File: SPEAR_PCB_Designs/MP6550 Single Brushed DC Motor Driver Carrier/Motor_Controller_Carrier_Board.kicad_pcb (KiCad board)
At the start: 2 copper layers, 104 x 47 mm, 21 parts, among them J1 Conn_01x02_Pin, J2 Conn_01x02_Pin, J3 Conn_01x02_Pin, J4 Conn_01x04_Pin, U1 AP63203WU

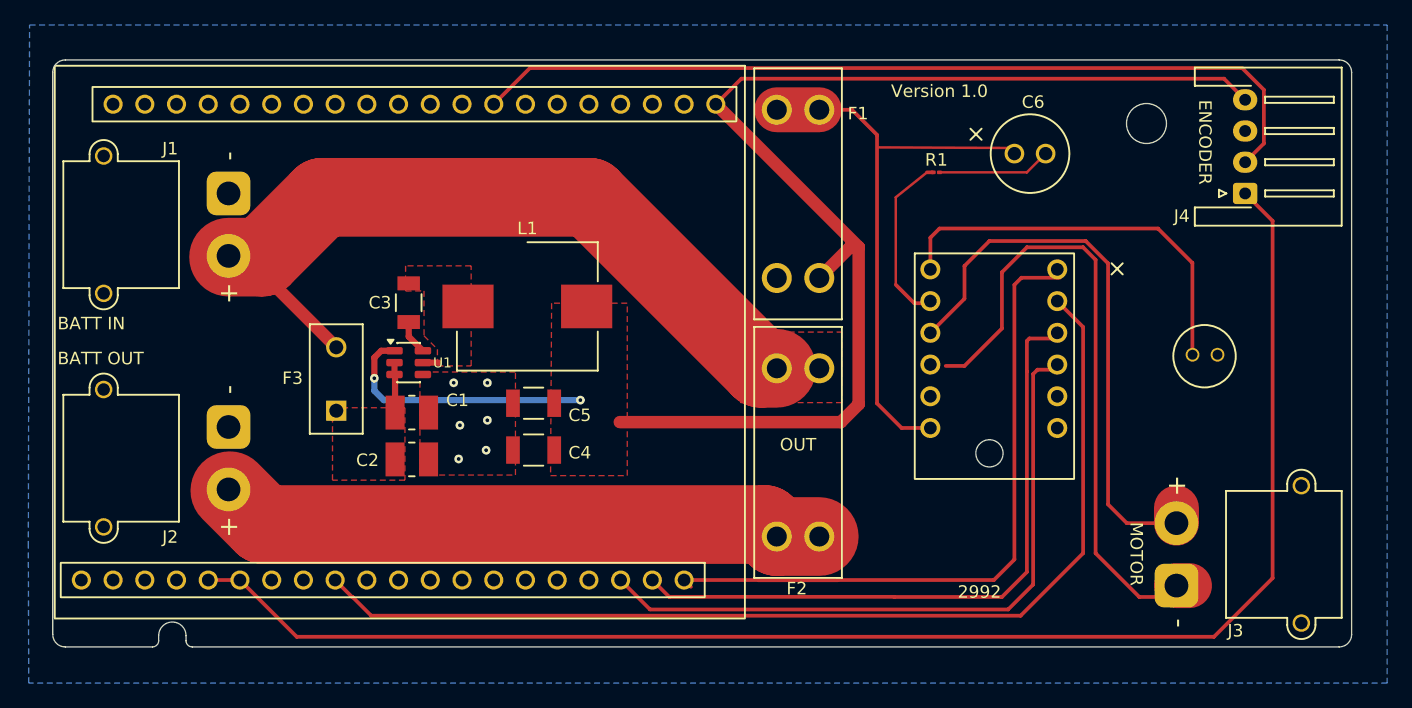
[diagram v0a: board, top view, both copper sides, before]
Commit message: update
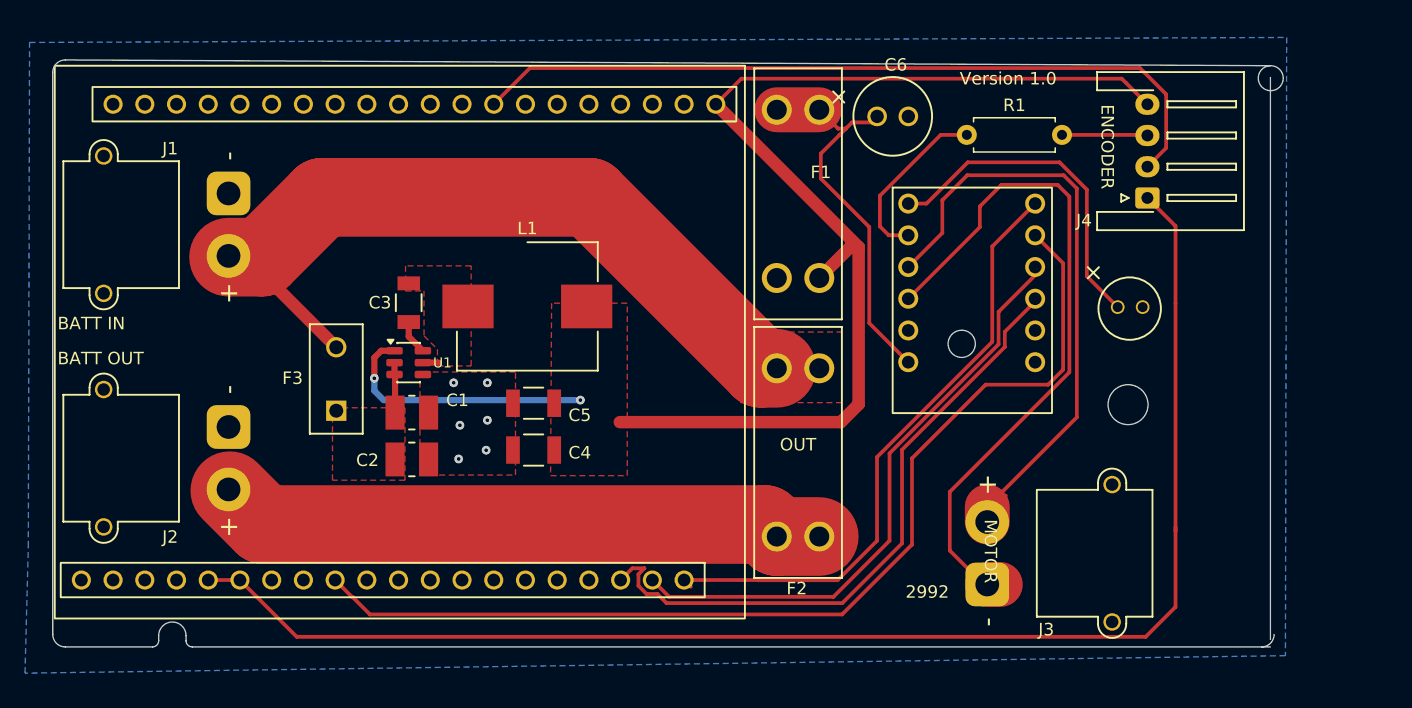
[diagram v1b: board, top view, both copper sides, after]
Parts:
- R1: footprint Resistor_SMD:R_01005_0402Metric -> Resistor_THT:R_Axial_DIN0207_L6.3mm_D2.5mm_P7.62mm_Horizontal
- moved REF** 22.6 mm to (171.1, 96.6)
- moved J3 15.2 mm to (159.8, 111.0)
- moved C6 11.4 mm to (148.5, 73.5)
- moved J4 7.83 mm to (172.7, 80.0)
- moved C7 7.10 mm to (173.4, 88.8)
- moved MDB1 5.56 mm to (152.2, 79.2)
- moved R1 3.87 mm to (158.2, 75.0)
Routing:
- net Net-(MDB1-ISET): track 4.20 -> 14.3 mm
- net +3.3V: track 117.7 -> 110.0 mm
- net /Schematic/ENC_A: track 70.0 -> 62.3 mm
- net GND: track 0.00 -> 6.86 mm
- net /Schematic/ENC_B: track 120.8 -> 114.4 mm
- net Net-(J3-Pin_1): track 51.8 -> 57.6 mm
- net Net-(MDB1-V3P3): track 32.7 -> 27.0 mm
- net Net-(J3-Pin_2): track 46.5 -> 51.4 mm
- net Net-(MDB1-VIN): track 35.4 -> 31.5 mm
- net /Schematic/PWM2: track 52.6 -> 48.8 mm
- net /Schematic/GPIO: track 53.8 -> 50.7 mm
- net /Schematic/PWM1: track 53.9 -> 51.4 mm
- net /Schematic/ADC: track 84.2 -> 83.3 mm
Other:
- board size 104 x 47 mm -> 98.5 x 47 mm

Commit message: updates
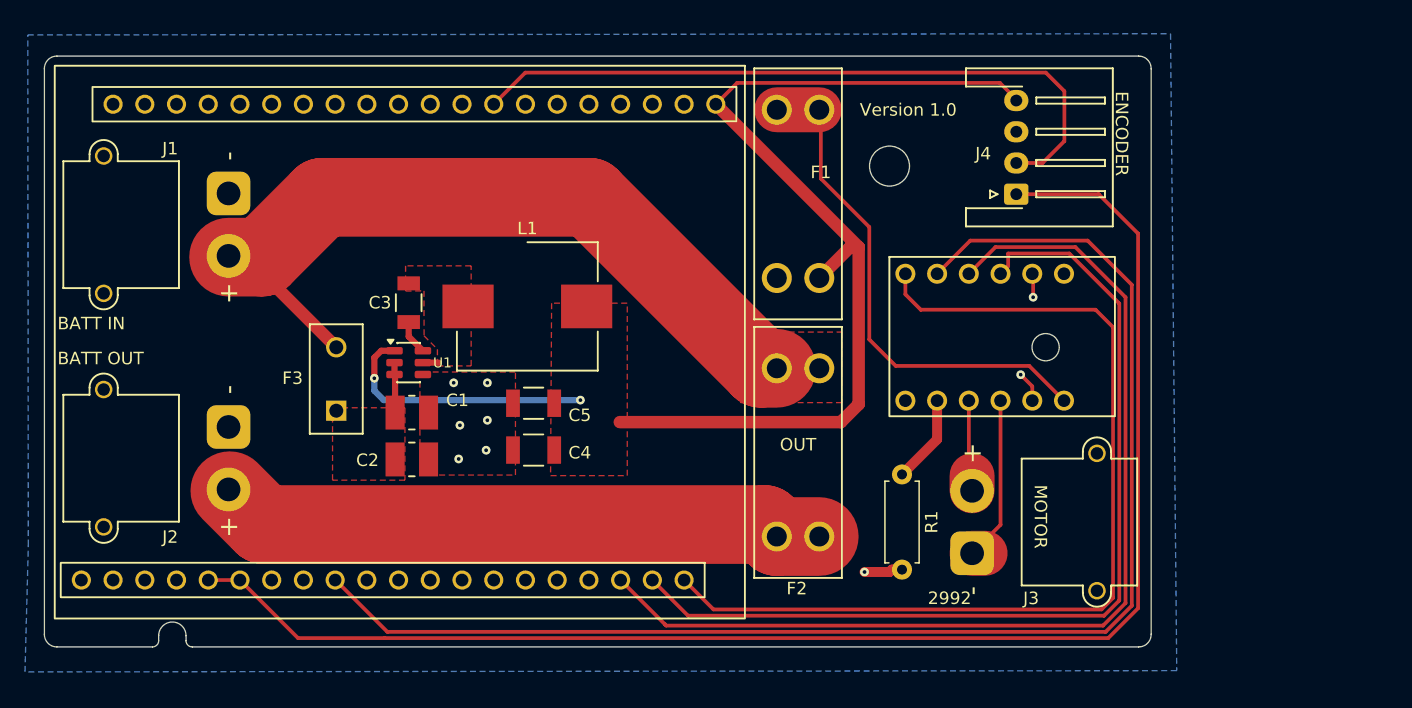
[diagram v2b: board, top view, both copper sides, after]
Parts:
- removed C6: 47uF, Motor_Controller_Carrier_Board:CAP_UBY_6.3X11_NCH
- removed C7: 0.47uF, Motor_Controller_Carrier_Board:CAP_UBY_18X20_NCH
- moved R1 27.7 mm to (153.0, 102.2), turned to -90 degrees
- moved REF** 27.0 mm to (152.0, 77.5)
- moved J4 10.5 mm to (162.2, 79.8)
- moved MDB1 3.92 mm to (154.6, 82.4)
- moved J3 2.78 mm to (158.6, 108.5)
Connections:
- MCB1 pad 22: /Schematic/PWM2 -> /Schematic/PWM1
- MCB1 pad 23: /Schematic/PWM1 -> /Schematic/PWM2
- MCB1 pad 31: /Schematic/CS -> unconnected-(MCB1-PB1-Pad31)
- MDB1 pad 6: Net-(MDB1-V3P3) -> GND
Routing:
- net Net-(J3-Pin_2): track 51.4 -> 5.37 mm
- net Net-(J3-Pin_1): track 57.6 -> 15.5 mm
- net /Schematic/PWM2: track 48.8 -> 82.3 mm
- net Net-(MDB1-V3P3): track 27.0 -> 0.00 mm
- net /Schematic/ADC: track 83.3 -> 110.2 mm
- net /Schematic/GPIO: track 50.7 -> 77.0 mm
- net /Schematic/PWM1: track 51.4 -> 75.3 mm
- net +3.3V: track 110.0 -> 99.2 mm
- net Net-(MDB1-VIN): track 31.5 -> 41.1 mm
- net Net-(MDB1-ISET): track 14.3 -> 7.07 mm
- net /Schematic/ENC_A: track 62.3 -> 56.4 mm
- net /Schematic/ENC_B: track 114.4 -> 118.8 mm
- net GND: track 6.86 -> 7.45 mm, vias 6 -> 9
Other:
- board size 98.5 x 47 mm -> 88.6 x 47.3 mm
